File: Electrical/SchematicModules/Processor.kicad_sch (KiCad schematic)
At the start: 30 parts, among them J1 3220-14-0300-00, SW1 DS04-254-2L-01BK, SW2 TS04-66-65-BK-160-SMT, SW3 TS04-66-65-BK-160-SMT, SW4 TS04-66-65-BK-160-SMT, SW5 TS04-66-65-BK-160-SMT, SW6 TS04-66-65-BK-160-SMT, SW7 TS04-66-65-BK-160-SMT, U1 STM32F103T6Ux, Y1 16 MHz

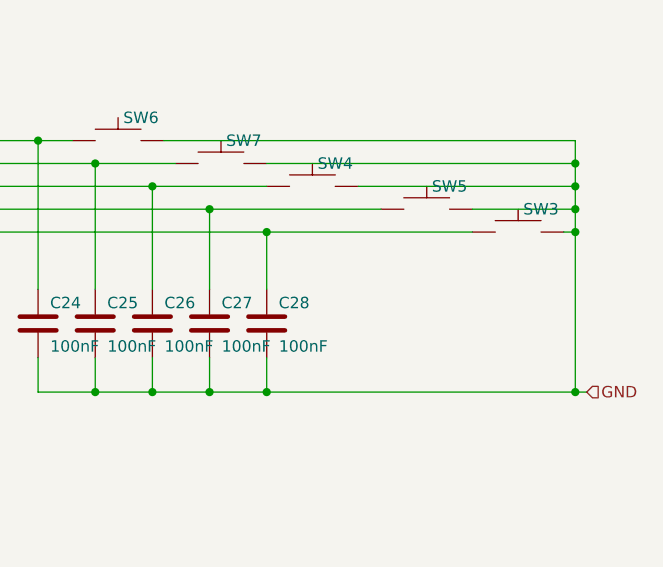
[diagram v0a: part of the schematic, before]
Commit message: Finalizing the layout
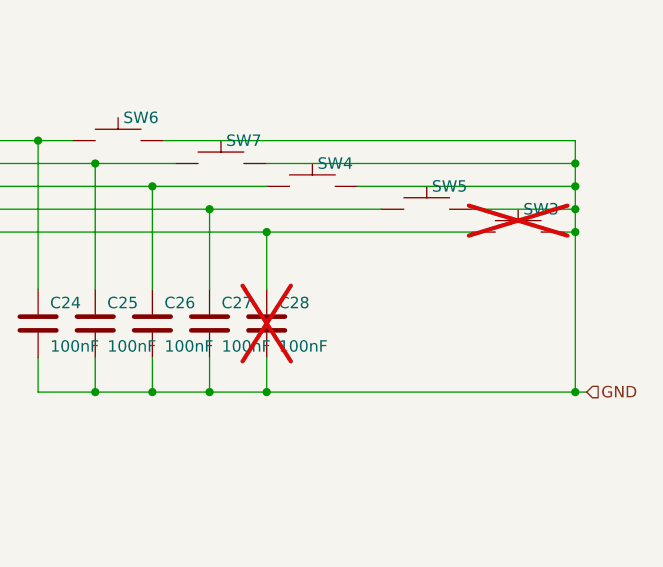
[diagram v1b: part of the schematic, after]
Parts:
- C28: now not fitted
- SW3: value TS04-66-65-BK-160-SMT -> TS04-66-95-BK-260-SMT; now not fitted
- SW4, SW5, SW6, SW7: value TS04-66-65-BK-160-SMT -> TS04-66-95-BK-260-SMT
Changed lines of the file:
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@@
 			)
 		)
-		(property "Value" "TS04-66-65-BK-160-SMT"
+		(property "Value" "TS04-66-95-BK-260-SMT"
 			(at 243.84 82.55 0)
 			(effects
@@
 			)
 		)
-		(property "Value" "TS04-66-65-BK-160-SMT"
+		(property "Value" "TS04-66-95-BK-260-SMT"
 			(at 222.25 77.47 0)
 			(effects
@@
 			)
 		)
-		(property "Value" "TS04-66-65-BK-160-SMT"
+		(property "Value" "TS04-66-95-BK-260-SMT"
 			(at 256.54 85.09 0)
 			(effects
@@
 			)
 		)
-		(property "Value" "TS04-66-65-BK-160-SMT"
+		(property "Value" "TS04-66-95-BK-260-SMT"
 			(at 233.68 80.01 0)
 			(effects
@@
 		(exclude_from_sim no)
 		(in_bom yes)
-		(on_board yes)
-		(dnp no)
+		(on_board no)
+		(dnp yes)
 		(property "Reference" "SW3"
 			(at 269.24 82.55 0)
@@
 			)
 		)
-		(property "Value" "TS04-66-65-BK-160-SMT"
+		(property "Value" "TS04-66-95-BK-260-SMT"
 			(at 266.7 87.63 0)
 			(effects
@@
 		(in_bom yes)
 		(on_board yes)
-		(dnp no)
+		(dnp yes)
 		(property "Reference" "C28"
 			(at 241.808 92.964 0)
